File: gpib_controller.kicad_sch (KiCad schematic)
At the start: 0 parts

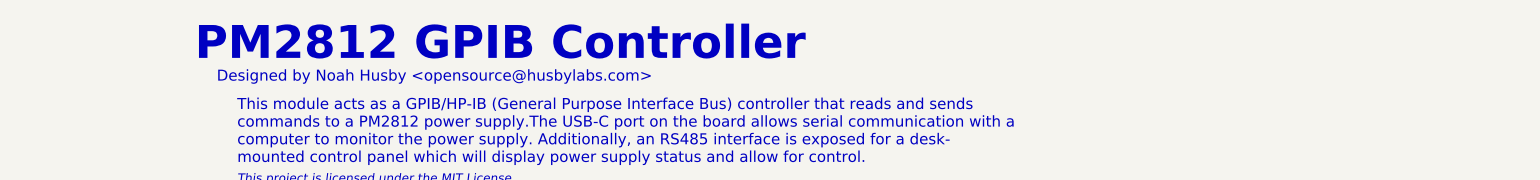
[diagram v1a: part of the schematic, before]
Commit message: Update name
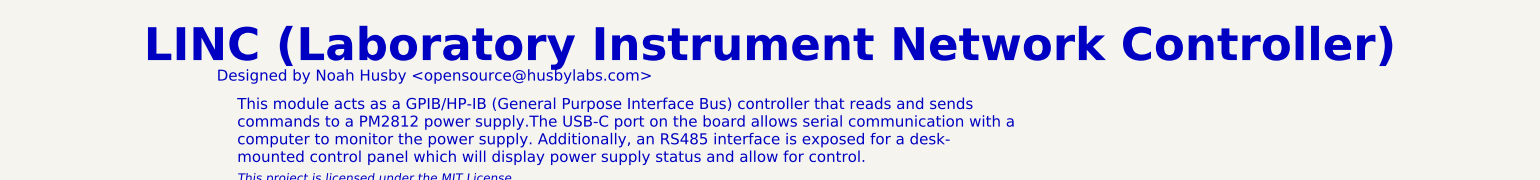
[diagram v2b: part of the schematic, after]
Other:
- note added: "LINC (Laboratory Instrument Network Controller)"
- note removed: "PM2812 GPIB Controller"
- title: (none) -> Project Overview
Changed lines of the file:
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@@
 	(paper "User" 431.8 279.4)
 	(title_block
-		(date "2026-03-12")
-		(rev "1")
+		(title "Project Overview")
+		(date "2026-03-27")
+		(rev "0.1")
 	)
 	(text "This project is licensed under the MIT License\nView license: https://opensource.org/license/mit"
@@
 		)
 	)
-	(text "PM2812 GPIB Controller"
+	(text "LINC (Laboratory Instrument Network Controller)"
 		(exclude_from_sim no)
-		(at 86.36 33.02 0)
+		(at 148.844 33.528 0)
 		(effects
 			(font
